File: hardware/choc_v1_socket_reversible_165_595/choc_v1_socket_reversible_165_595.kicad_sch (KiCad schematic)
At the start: 70 parts, among them SW00 SW_Push, SW01 SW_Push, SW02 SW_Push, SW03 SW_Push, SW04 SW_Push, SW05 SW_Push, SW10 SW_Push, SW11 SW_Push, SW12 SW_Push, SW13 SW_Push, SW14 SW_Push, SW15 SW_Push, SW20 SW_Push, SW21 SW_Push, SW22 SW_Push, SW23 SW_Push, SW24 SW_Push, SW25 SW_Push, SW26 SW_Push, SW30 SW_Push, SW31 SW_Push, SW32 SW_Push, SW33 SW_Push, SW34 SW_Push, SW35 SW_Push, SW36 SW_Push, U1 CH582

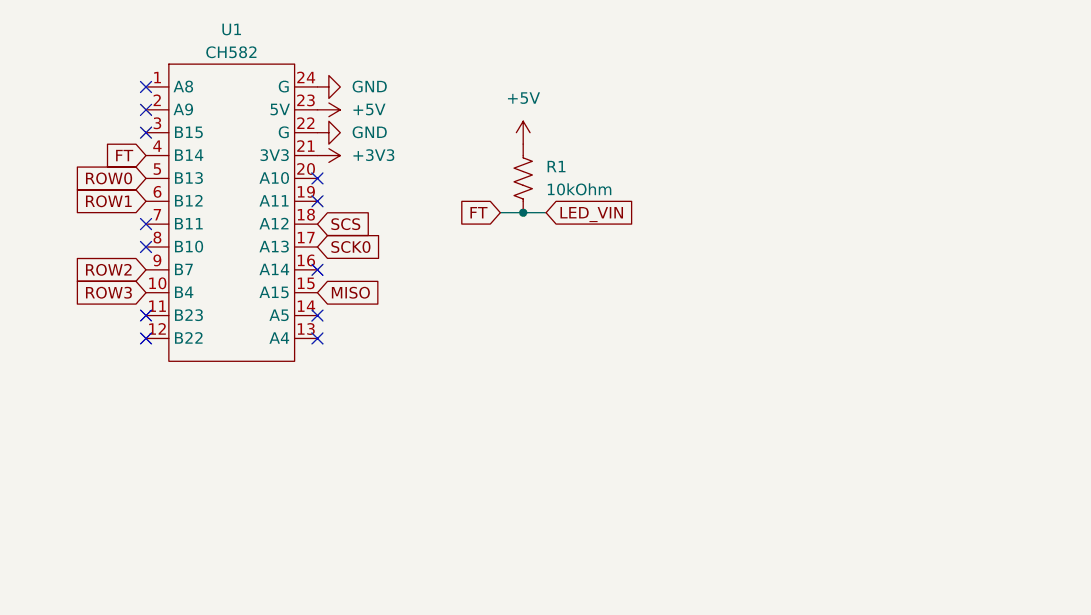
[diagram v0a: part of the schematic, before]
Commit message: Finished layout
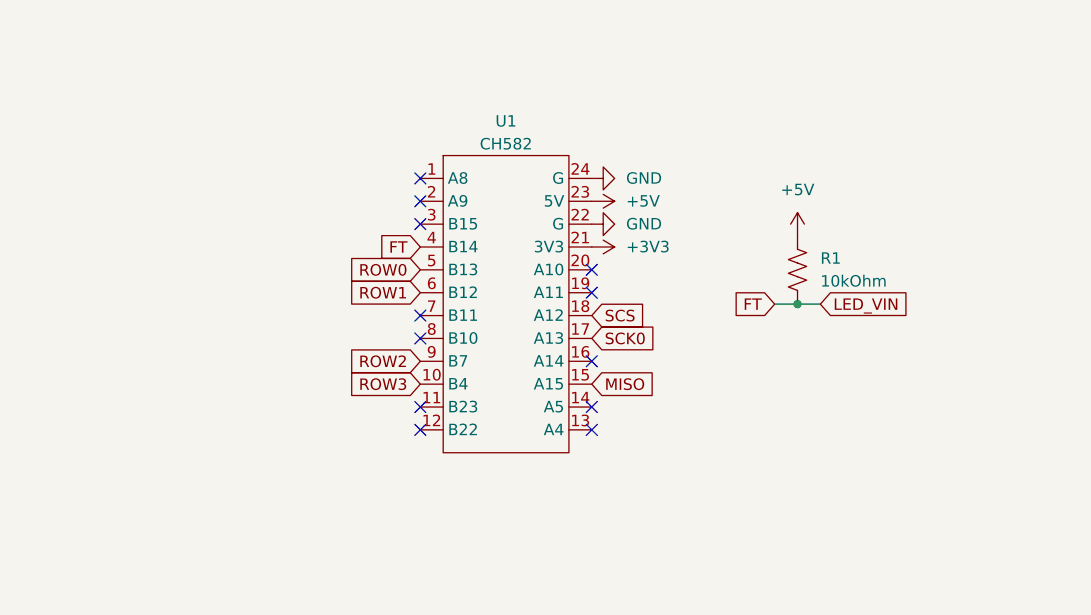
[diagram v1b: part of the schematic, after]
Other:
- moved on the sheet: R1, U1
